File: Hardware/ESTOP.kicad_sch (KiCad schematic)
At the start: 28 parts, among them J10 Conn_01x02, Q13 SQ2315CES-T1_GE3, Q15 IRLML0030, Q16 IRLML0030, Q17 IRLML0030, Q7 SQ2315CES-T1_GE3, Q8 SQ2315CES-T1_GE3

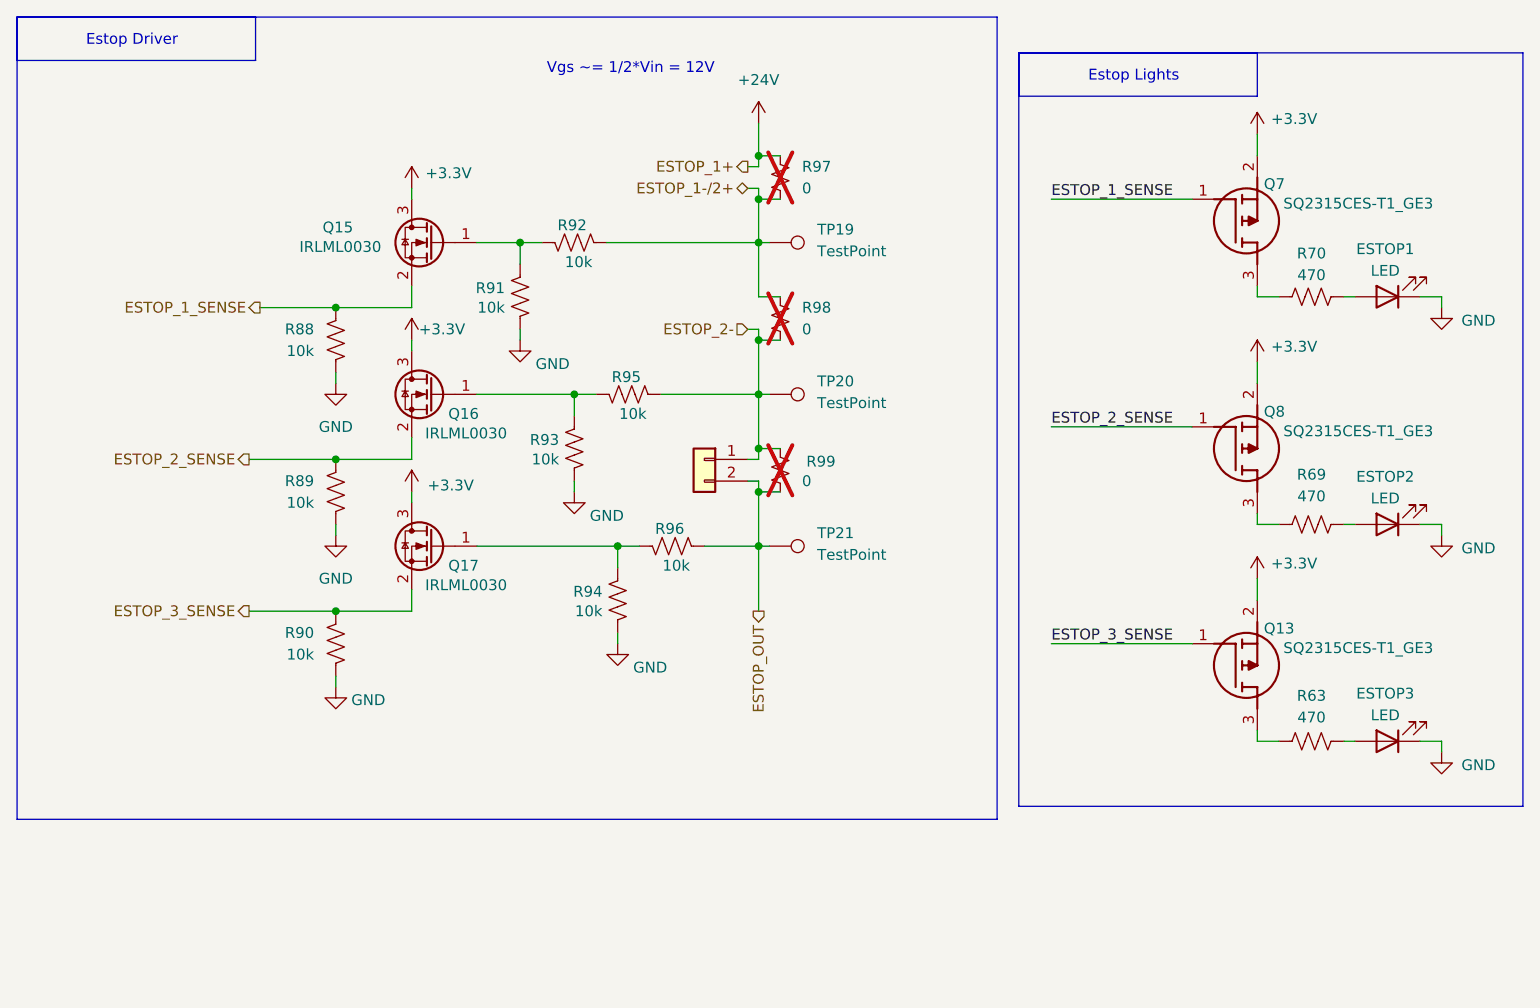
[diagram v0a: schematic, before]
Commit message: circuit blocks designed, schematic updated
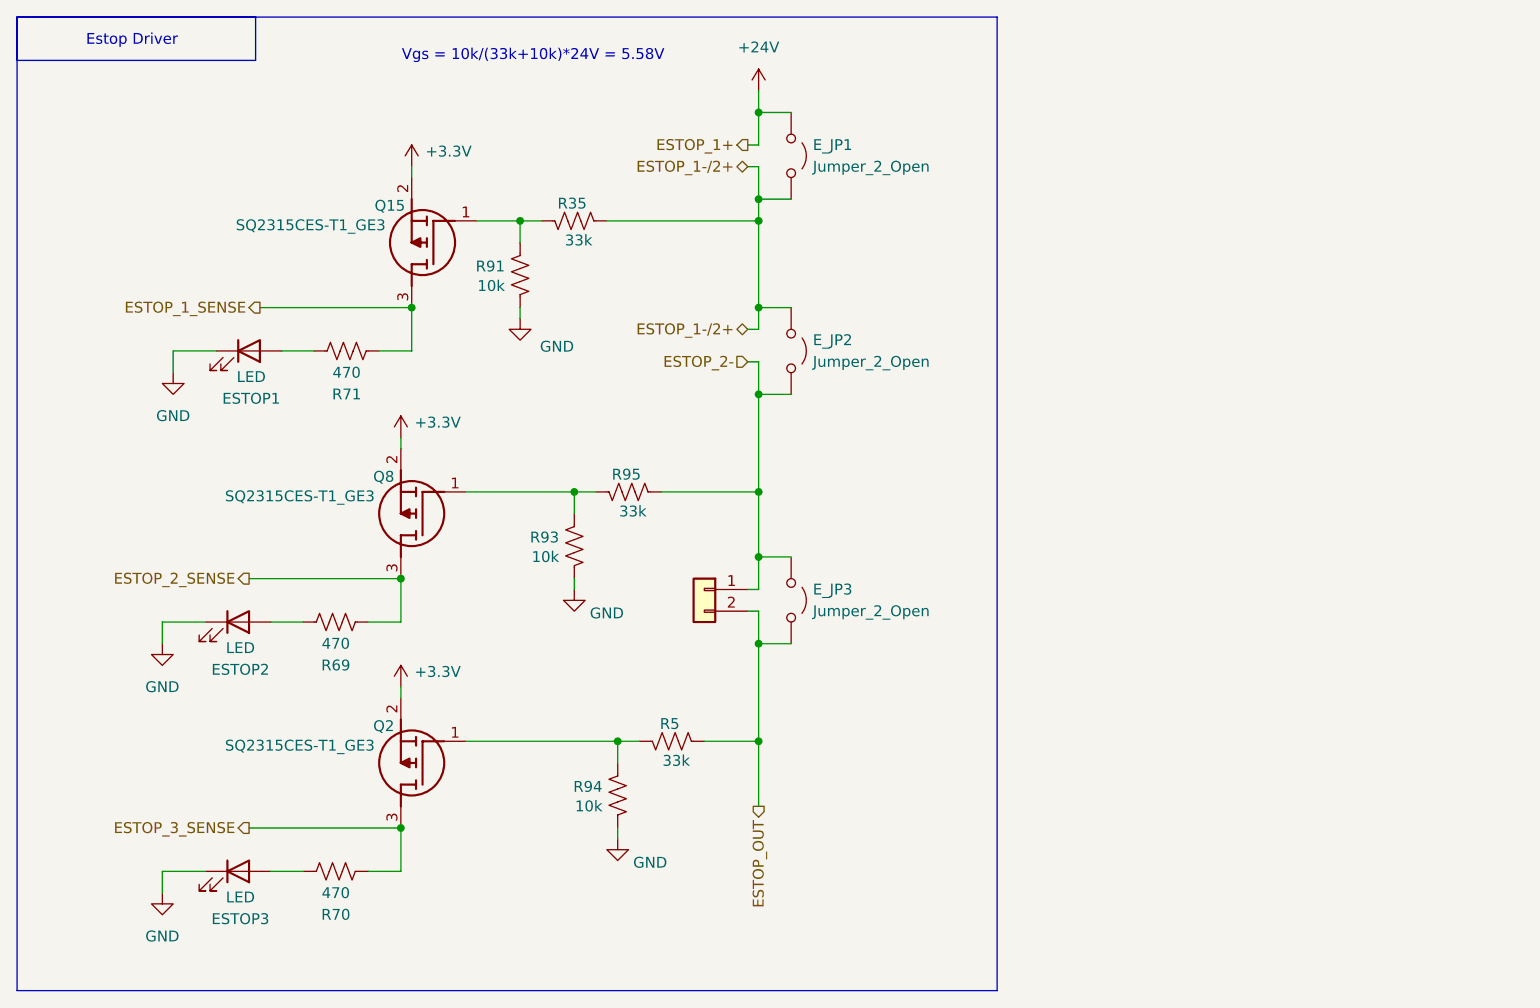
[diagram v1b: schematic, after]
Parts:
- removed Q13, Q7: SQ2315CES-T1_GE3, SQ2315CES-T1_GE3:SOT95P237X112-3N, symbol SQ2315CES-T1_GE3:SQ2315CES-T1_GE3
- removed Q15, Q16, Q17: IRLML0030, Package_TO_SOT_SMD:SOT-23, symbol Transistor_FET:IRLML0030
- removed R63: 470, Resistor_SMD:R_0603_1608Metric, symbol Device:R_US
- removed R88, R89, R90, R92, R96: 10k, Resistor_SMD:R_0603_1608Metric, symbol Device:R_US
- removed R97, R98, R99: 0, Resistor_SMD:R_0603_1608Metric, symbol Device:R_Small_US
- removed TP19, TP20, TP21: TestPoint, TestPoint:TestPoint_Pad_1.0x1.0mm, symbol Connector:TestPoint
- added E_JP1, E_JP2, E_JP3: Jumper_2_Open, Connector_PinHeader_2.54mm:PinHeader_1x02_P2.54mm_Vertical, symbol Jumper:Jumper_2_Open
- added Q15, Q2: SQ2315CES-T1_GE3, SQ2315CES-T1_GE3:SOT95P237X112-3N, symbol SQ2315CES-T1_GE3:SQ2315CES-T1_GE3
- added R35, R5: 33k, Resistor_SMD:R_0603_1608Metric, symbol Device:R_US
- added R71: 470, Resistor_SMD:R_0603_1608Metric, symbol Device:R_US
- R95: value 10k -> 33k
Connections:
- net +24V: now also E_JP1.1 (A)
- net +3.3V: now also Q15.2 (S), Q2.2 (S)
- net ESTOP_1-/2+: now also E_JP1.2 (B), E_JP2.1 (A), R35.2
- net ESTOP_1_SENSE: now also Q15.3 (D), R71.1
- net ESTOP_2-: now also E_JP2.2 (B), E_JP3.1 (A)
- net ESTOP_2_SENSE: now also Q8.3 (D), R69.1; no longer Q8.1 (G)
- net ESTOP_3_SENSE: now also R70.1, Q2.3 (D)
- net ESTOP_OUT: now also E_JP3.2 (B), R5.2
- net at ESTOP1.2 (A): now also R71.2; no longer R70.2
- net at R93.2, R95.1: now also Q8.1 (G)
- net at ESTOP3.2 (A): now also R70.2
- net at R94.2: now also Q2.1 (G), R5.1
- net at R91.2: now also Q15.1 (G), R35.1
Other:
- note added: "Vgs = 10k/(33k+10k)*24V = 5.58V"
- note removed: "Estop Lights"
- note removed: "Vgs ~= 1/2*Vin = 12V"
- moved on the sheet: R91, R93, R94, R95
